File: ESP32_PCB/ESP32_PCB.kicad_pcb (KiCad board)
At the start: 2 copper layers, 35 x 35 mm, 35 parts, among them J1 USB_C_Receptacle, J2 ESC 1, J3 ESC 2, J4 EN & Boot, J5 LED, U2 H3LIS331DL, U3 AP2112K-3.3, U4 TPS54302, U5 ESP32-S3-MINI-1U

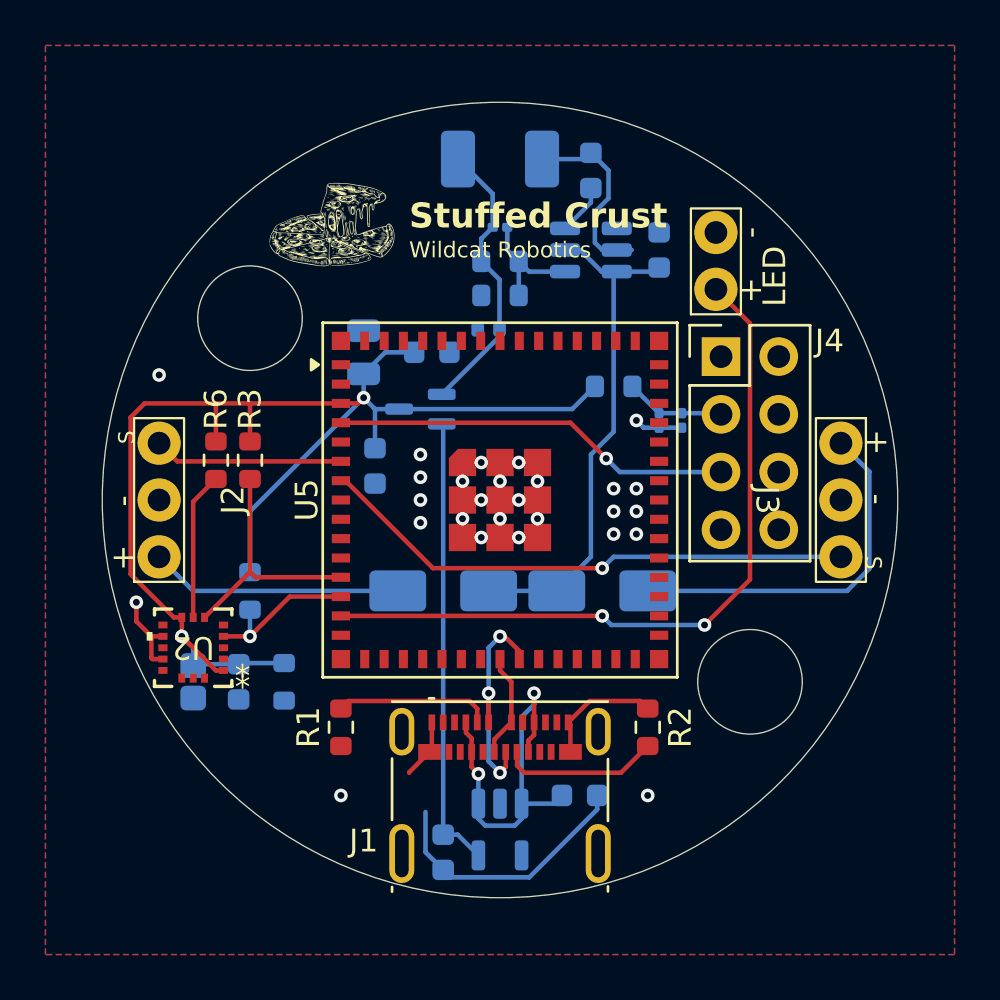
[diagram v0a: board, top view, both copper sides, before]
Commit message: rerouting
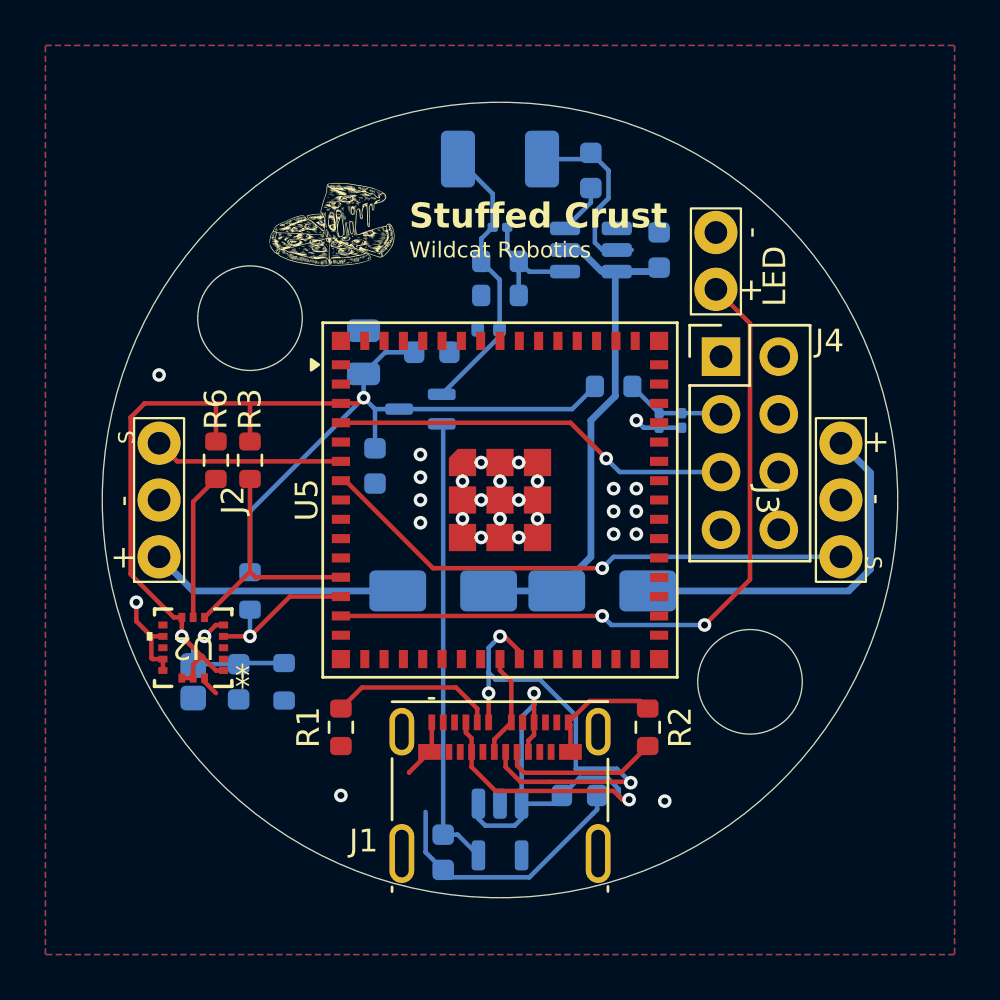
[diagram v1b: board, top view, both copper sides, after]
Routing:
- net /USB_D+: track 10.2 -> 21.5 mm
- net Net-(U3-EN): track 17.1 -> 27.0 mm
- net GNDREF: track 25.5 -> 27.9 mm, vias 27 -> 28
- net +3V3: track 58.7 -> 60.3 mm
